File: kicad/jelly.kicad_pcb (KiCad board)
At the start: 2 copper layers, 59.9 x 32.9 mm, 30 parts, among them M1 PAGER_MOTOR, M2 PAGER_MOTOR, P1 CONN_01X01, P10 CONN_01X01, P11 CONN_01X01, P12 CONN_01X01, P13 CONN_01X01, P14 CONN_01X01, P15 CONN_01X01, P2 CONN_01X01, P3 CONN_01X01, P4 CONN_01X01, P5 CONN_01X01, P6 CONN_01X01, P7 CONN_01X01, P8 CONN_01X01, P9 CONN_01X01, Q1 2N7000, Q2 2N7000

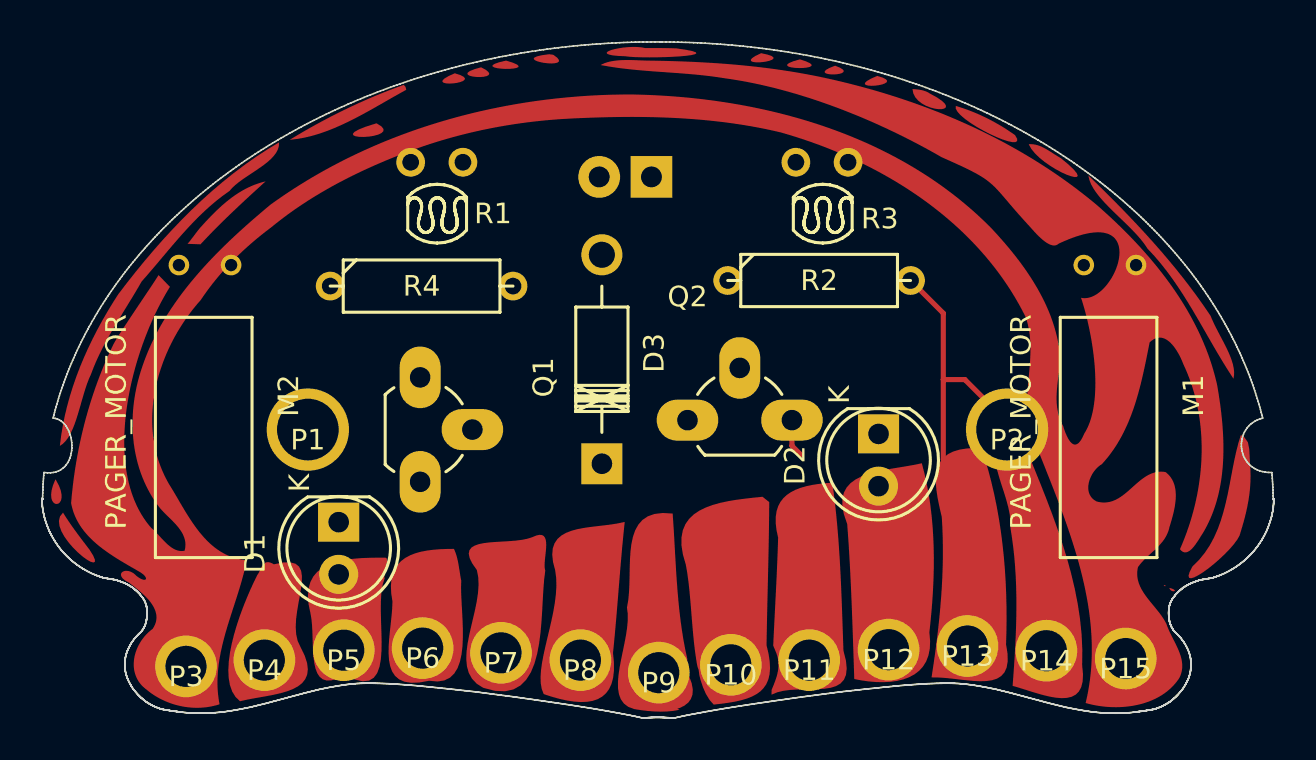
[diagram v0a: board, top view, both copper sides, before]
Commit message: Switch to low side switch and layout about
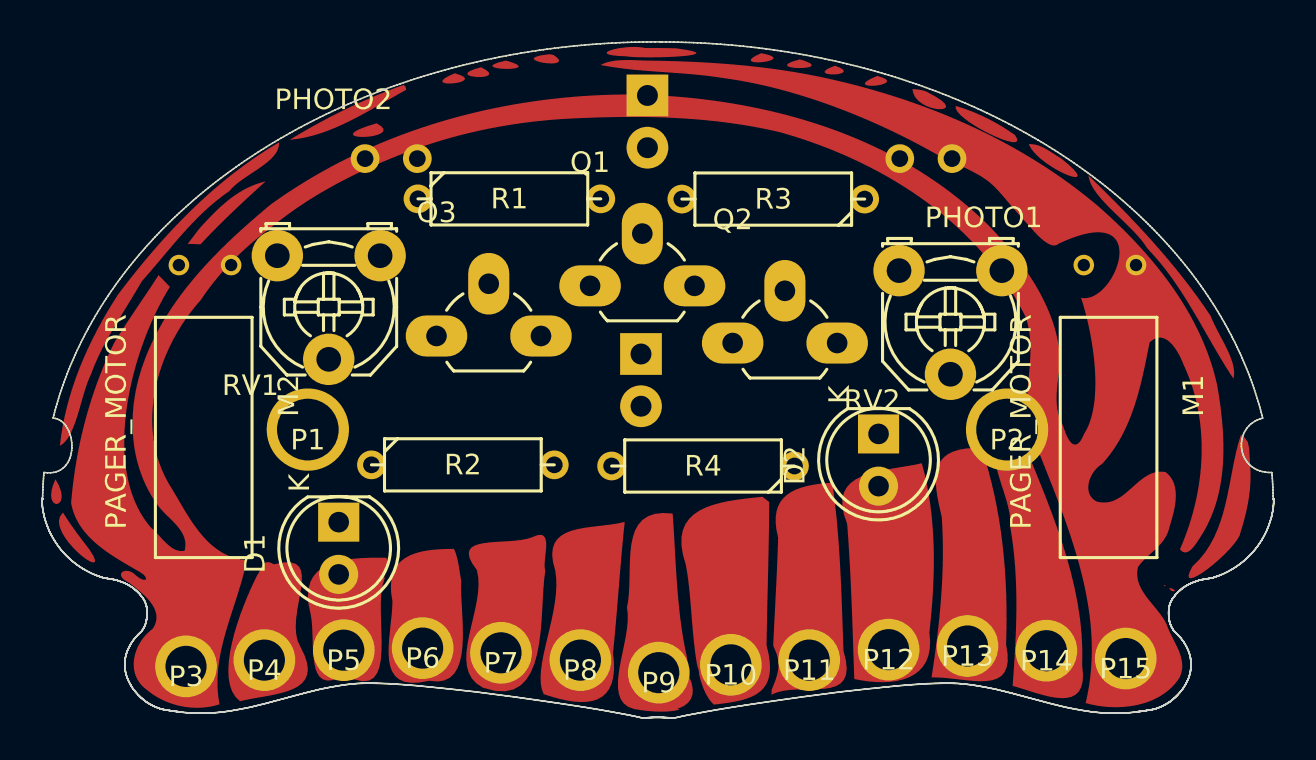
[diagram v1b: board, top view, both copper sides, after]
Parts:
- removed D3: D_Small, KiCad/Diodes_ThroughHole.pretty:Diode_DO-41_SOD81_Horizontal_RM10
- added PHOTO1: Photores, custom:ldr, F.Cu at (163.1, 69.8)
- added PHOTO2: Photores, custom:ldr, F.Cu at (137.1, 69.8)
- added Q3: Q_NMOS_SGD, KiCad/TO_SOT_Packages_THT.pretty:TO-92_Rugged, F.Cu at (139.3, 78.4)
- added RV1: POT, KiCad/Potentiometers.pretty:Potentiometer_Triwood_RM-065, F.Cu at (136.5, 74.5)
- added RV2: POT, KiCad/Potentiometers.pretty:Potentiometer_Triwood_RM-065, F.Cu at (166.7, 75.3)
- added SW1: SPST, KiCad/Pin_Headers.pretty:Pin_Header_Straight_1x02, B.Cu at (149.2, 79.3)
- DNP2, DNP3: moved to B.Cu
- Q1, Q2: value 2N7000 -> Q_NMOS_SGD
- R1: value Photores -> 1k; footprint custom:ldr -> KiCad/Discret.pretty:R3-5
- R2: value 220 -> 120
- R3: value Photores -> 100k; footprint custom:ldr -> KiCad/Discret.pretty:R3-5
- R4: value R -> 120
- moved R2 19.5 mm to (140.5, 84.7)
- moved R4 16.2 mm to (152.2, 84.8), turned to 180 degrees
- moved Q1 9.39 mm to (146.7, 76.0), turned to 0 degrees
- moved DNP3 5.06 mm to (163.1, 72.2)
- moved Q2 4.35 mm to (153.7, 78.8)
- moved BT1 3.97 mm to (149.5, 66.8), turned to 180 degrees
- moved R1 3.95 mm to (142.8, 71.8), turned to 0 degrees
- moved R3 2.97 mm to (155.6, 71.8), turned to 180 degrees
- moved DNP2 2.26 mm to (137.0, 72.2)
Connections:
- BT1 pad 1: Net-(BT1-Pad1) -> VCC
- BT1 pad 2: GND -> Net-(BT1-Pad2)
- M1 pad 2: Vout1 -> Vout2
- M2 pad 2: Vout2 -> Vout1
- Q1 pad 3: Vout1 -> Net-(BT1-Pad2)
- Q2 pad 2: Net-(Q2-Pad2) -> Net-(PHOTO2-Pad1)
- R1 pad 1: Net-(Q1-Pad2) -> Net-(R1-Pad1)
- R1 pad 2: VCC -> Net-(Q1-Pad2)
- R3 pad 1: Net-(Q2-Pad2) -> Net-(Q1-Pad2)
- R3 pad 2: VCC -> GND
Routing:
- net VCC: track 23.5 -> 0.48 mm
- net Vout2: track 1.90 -> 0.00 mm
